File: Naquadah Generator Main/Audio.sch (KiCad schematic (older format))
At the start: 56 parts, among them J5 Conn_01x07, J6 Conn_01x07, J7 Conn_01x04, U7 VS1000, U9 MX25L1606EM1I-12G, Y2 12MHz

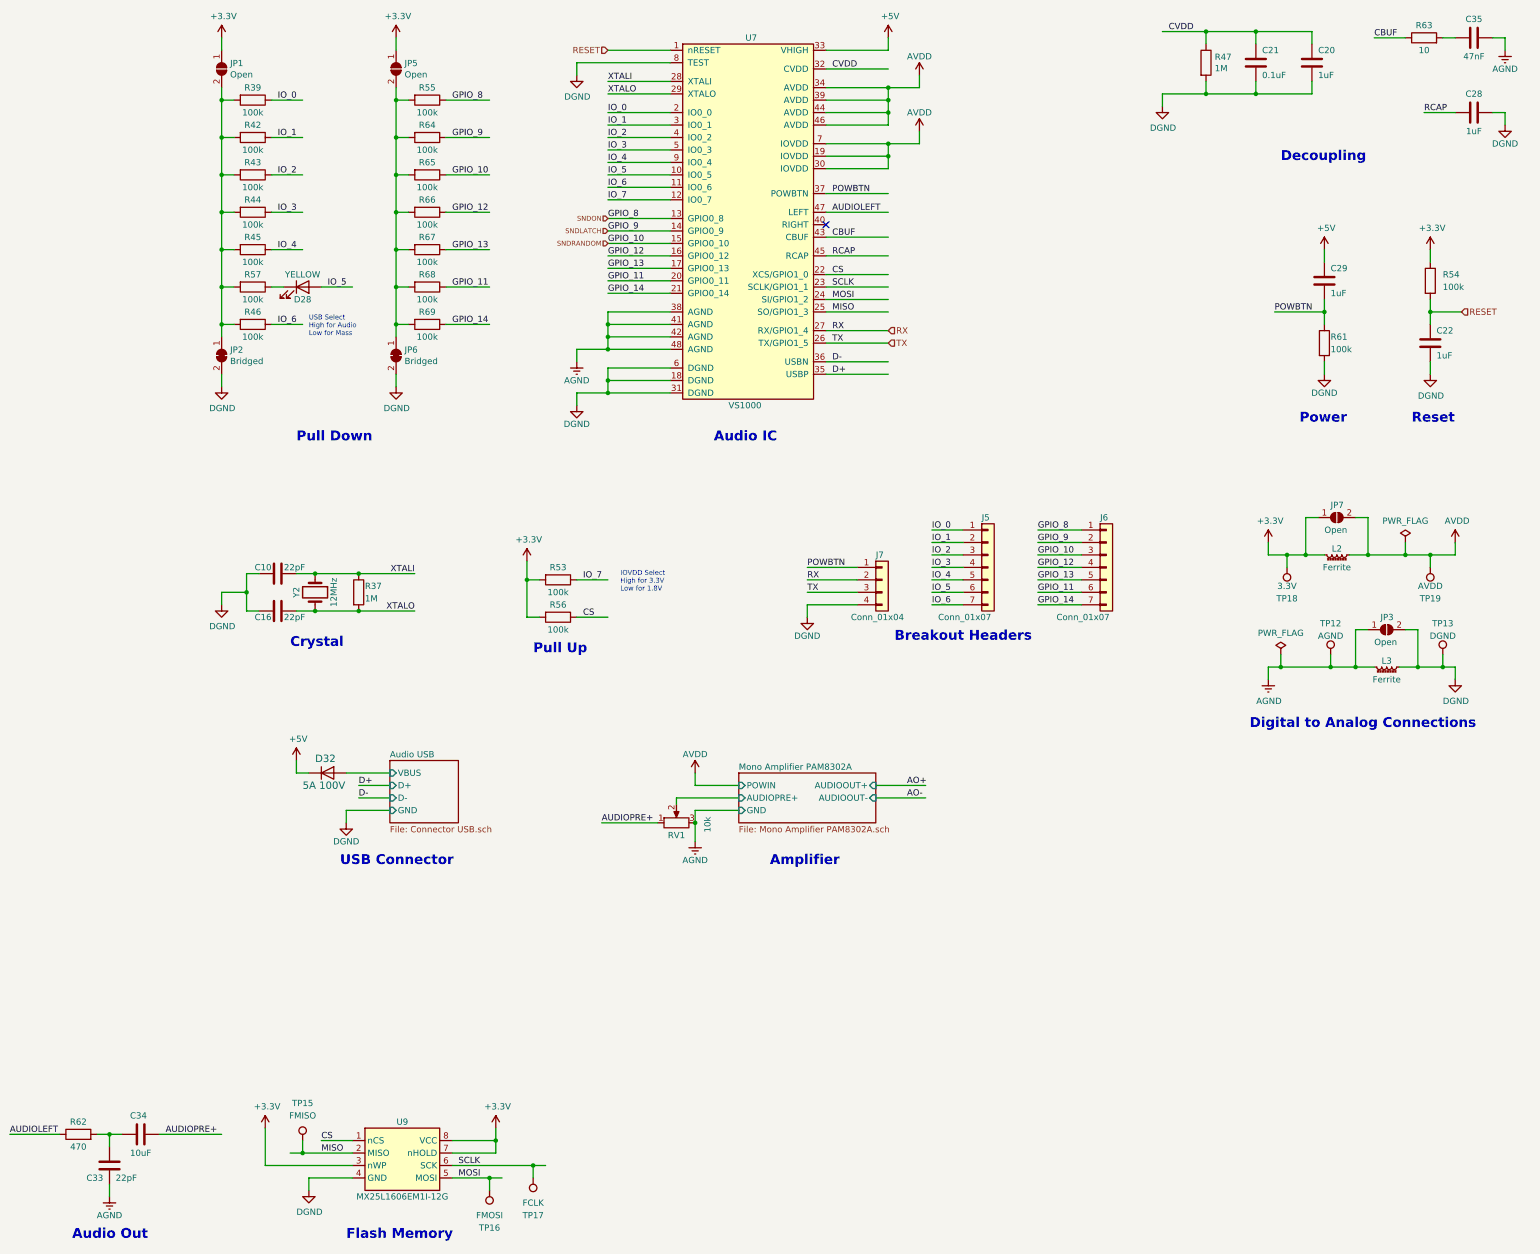
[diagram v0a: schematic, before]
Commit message: Clean up of audio page
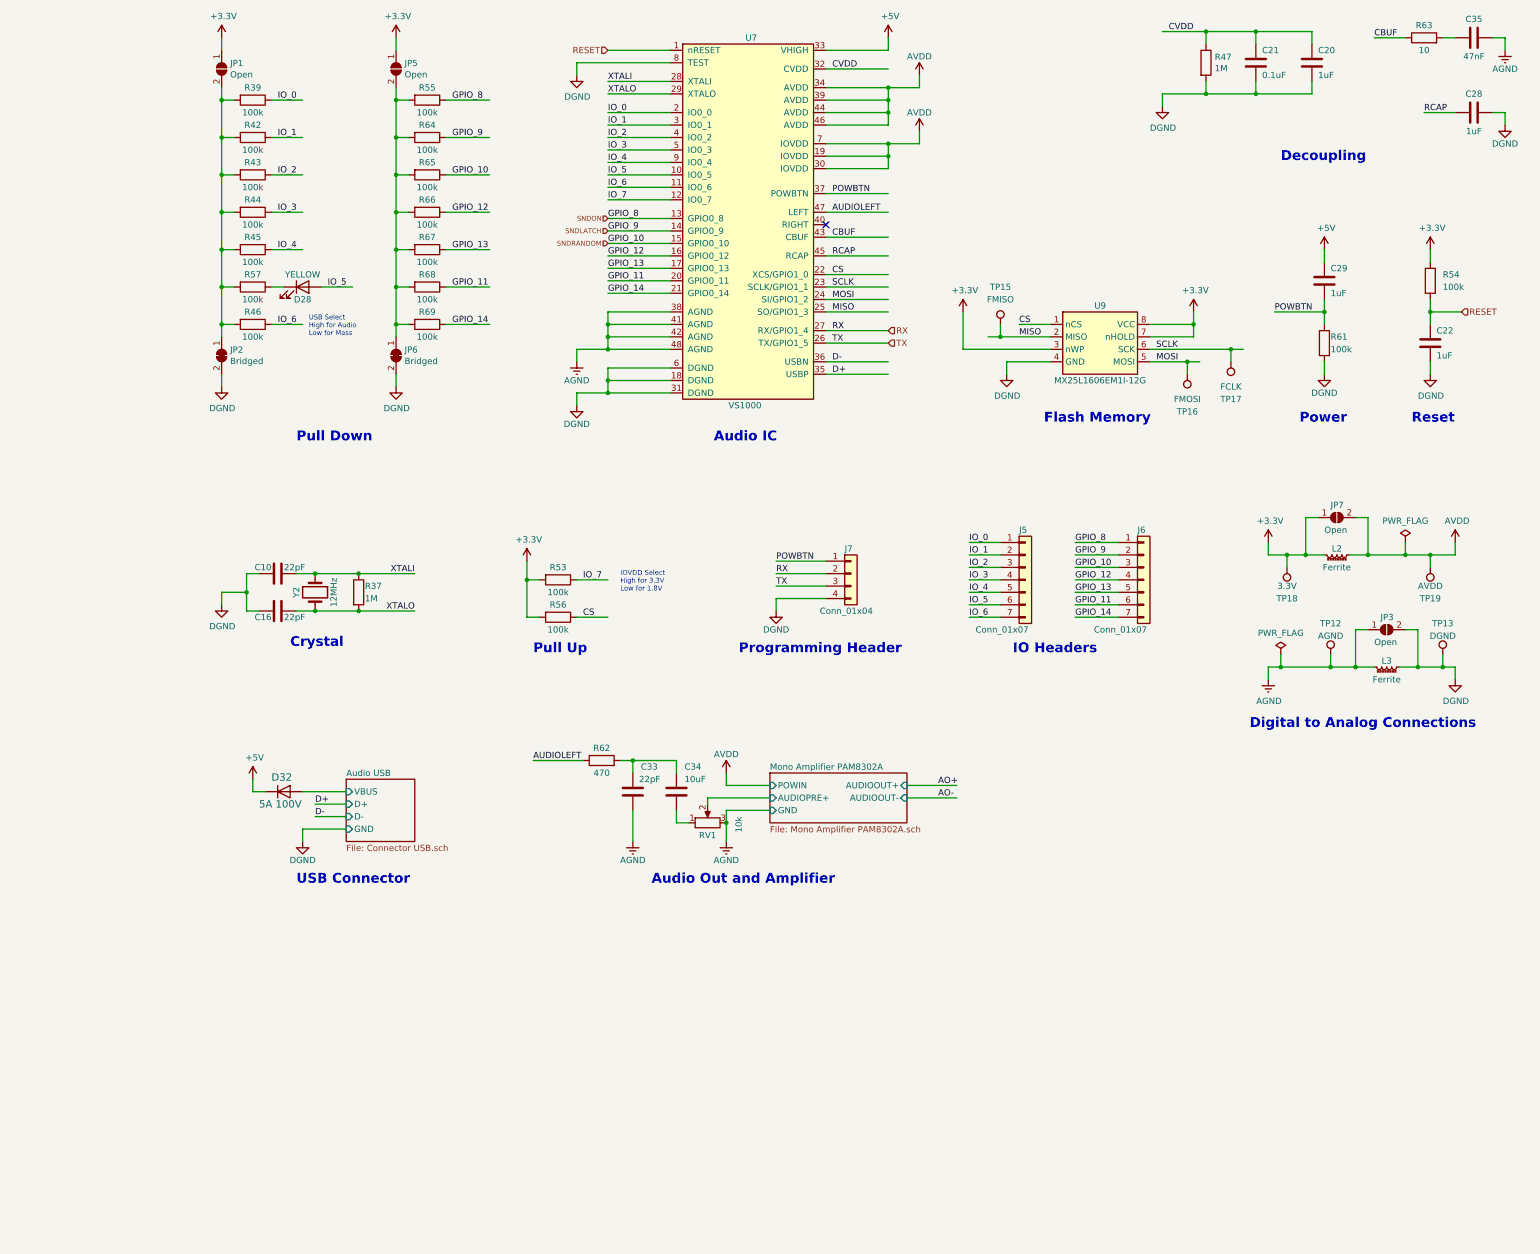
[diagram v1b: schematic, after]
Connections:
- net labels removed: AUDIOPRE+
- wire segments 256 -> 257
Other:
- note added: "Audio Out and Amplifier"
- note added: "IO Headers"
- note added: "Programming Header"
- note removed: "Amplifier"
- note removed: "Audio Out"
- note removed: "Breakout Headers"
- moved on the sheet: C33, C34, D32, J5, J6, J7, R62, RV1, TP15, TP16, TP17, U9
